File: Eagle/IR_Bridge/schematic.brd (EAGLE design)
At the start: 160 x 100 mm, 21 parts, among them T1 2N3904, T2 2N3904, T3 2N3904, T4 2N3904, T5 2N3904, T6 2N3904, T7 2N3904

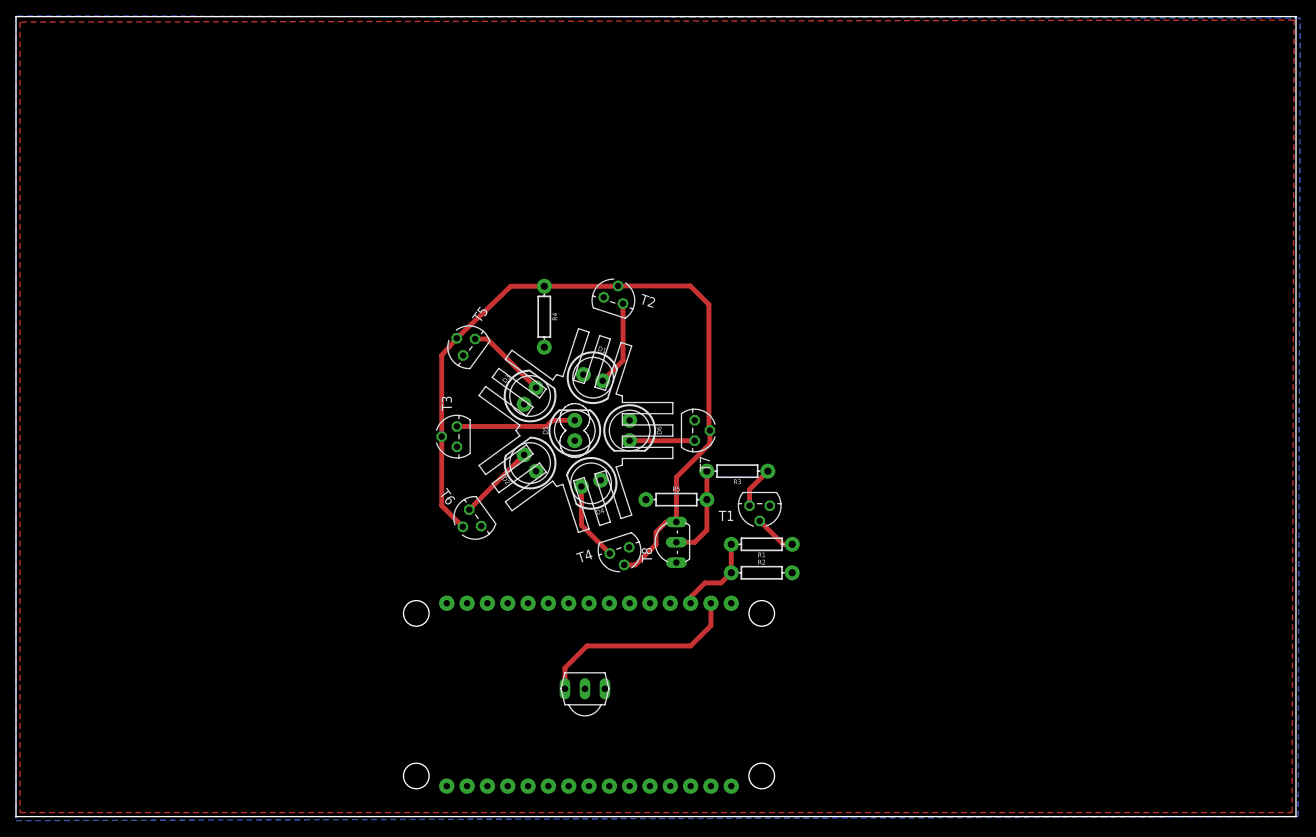
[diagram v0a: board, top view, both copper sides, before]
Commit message: Finish designing PCB
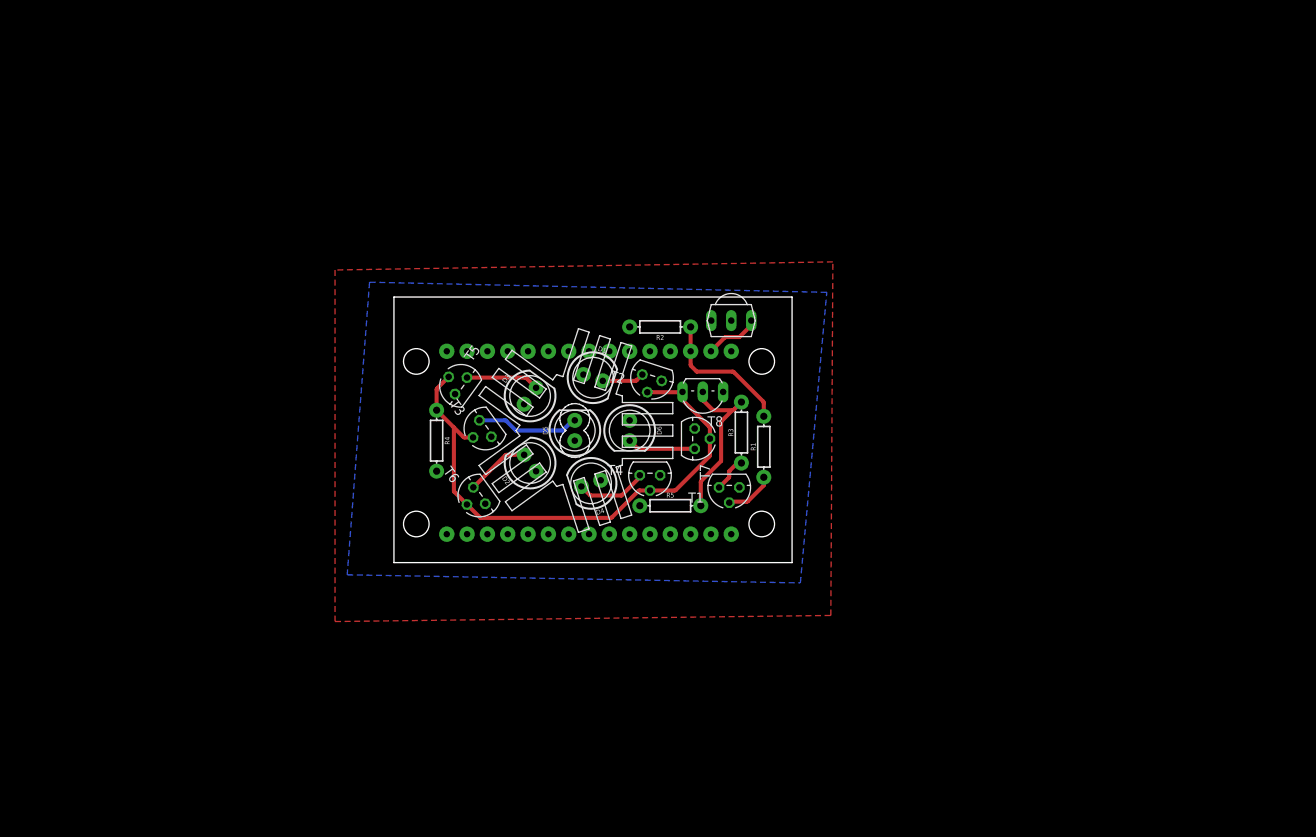
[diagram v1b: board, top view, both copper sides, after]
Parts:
- removed U$1: ESP12E_DEVKIT, ESP12E_DEVKIT:ESP12E_DEVKIT
- removed U$2: TSOP4838, tsop:TSOP18XX
- added NODEMCU: ESP12E_DEVKIT, ESP12E_DEVKIT:ESP12E_DEVKIT
- added RECEIVER: TSOP4838, tsop:TSOP18XX
- moved R2 33.3 mm to (10.7, 13.0), turned to 180 degrees
- moved R4 20.5 mm to (-17.3, -1.27)
- moved T8 18.1 mm to (16.0, 3.56), turned to 180 degrees
- moved R1 12.2 mm to (23.6, -2.03), turned to 90 degrees
- moved T2 10.8 mm to (9.65, 6.60), turned to 162 degrees
- moved T4 10.1 mm to (9.40, -5.59), turned to 180 degrees
- moved T5 4.93 mm to (-14.2, 5.59)
- moved R3 4.85 mm to (20.8, -0.25), turned to 90 degrees
- moved T1 4.44 mm to (19.3, -7.11)
- moved T3 3.70 mm to (-11.2, 0.25), turned to 126 degrees
- moved T6 2.84 mm to (-11.9, -8.13)
- moved R5 1.08 mm to (11.9, -9.40)
- moved T7 1.02 mm to (15.0, -1.02)
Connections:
- net +5V: now also NODEMCU.VIN, RECEIVER.VCC; no longer U$1.VIN, U$2.VCC
- net GND: now also NODEMCU.GND@3, RECEIVER.GND; no longer U$1.GND@3, U$2.GND
- net N$1: now also NODEMCU.D2; no longer U$1.D2
- net N$6: now also NODEMCU.D1, RECEIVER.OUT; no longer U$1.D1, U$2.OUT
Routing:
- net N$2: track 99.2 -> 69.0 mm
- net N$6: track 25.8 -> 6.93 mm
- net N$5: track 11.8 -> 20.3 mm
- net N$1: track 10.7 -> 17.6 mm
- net N$10: track 10.7 -> 5.26 mm
- net N$14: track 15.0 -> 12.9 mm
- net N$11: track 9.70 -> 8.02 mm
- net N$12: track 10.1 -> 9.15 mm
- net N$3: track 5.27 -> 6.20 mm
- net N$13: track 9.85 -> 8.94 mm
- net N$4: track 5.26 -> 4.47 mm
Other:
- board size 160 x 100 mm -> 49.8 x 33.2 mm
